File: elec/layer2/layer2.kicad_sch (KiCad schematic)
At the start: 24 parts, among them U4 DEV-15583

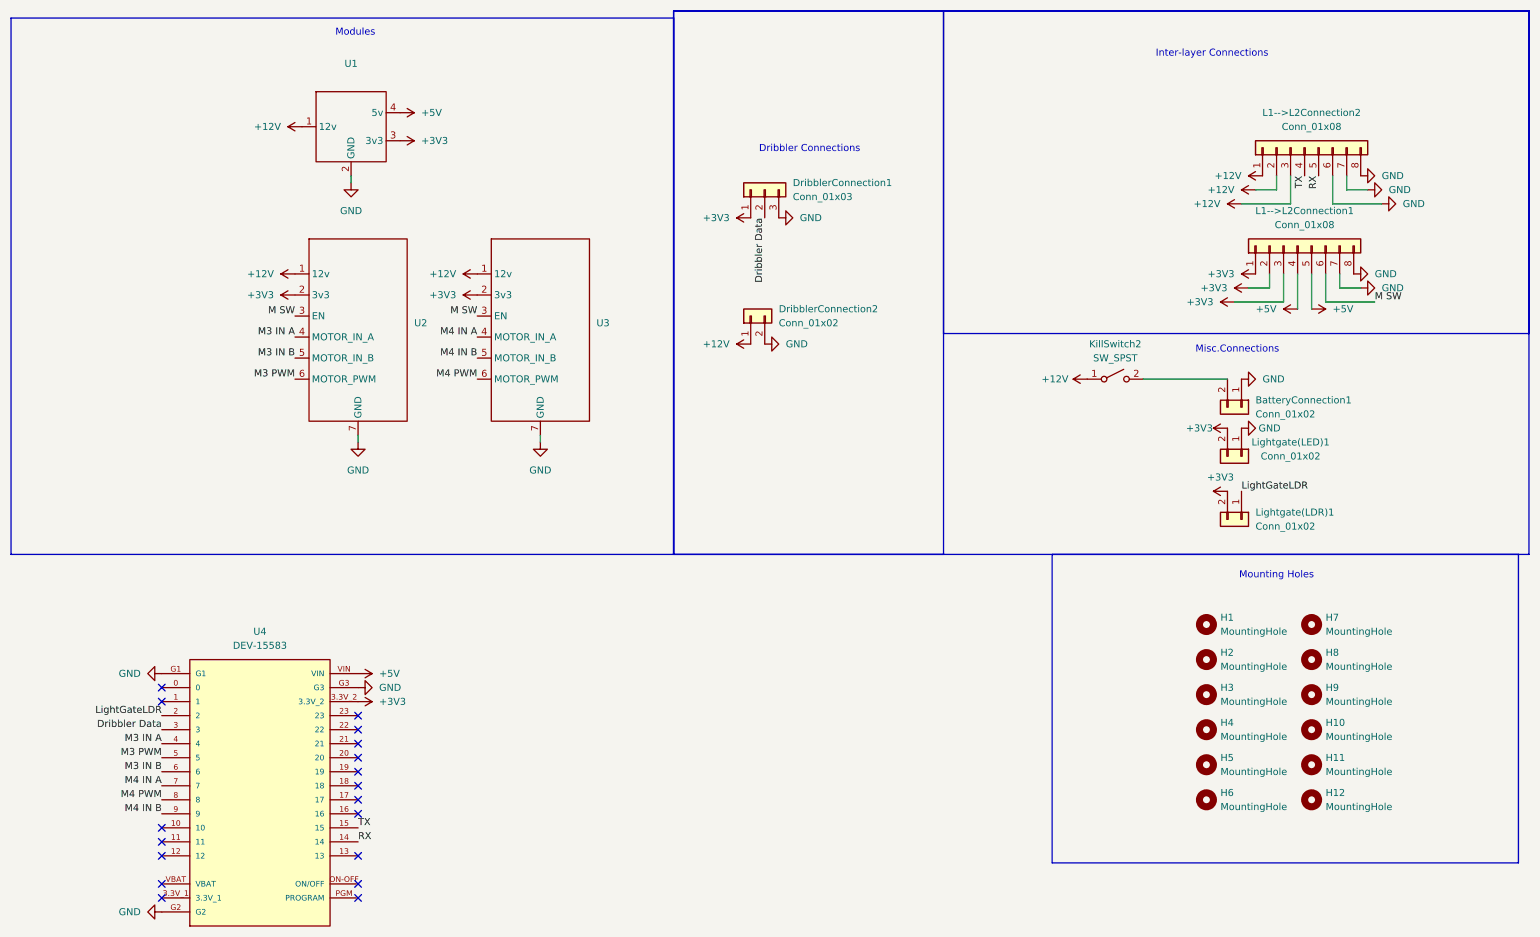
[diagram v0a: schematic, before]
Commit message: stuff
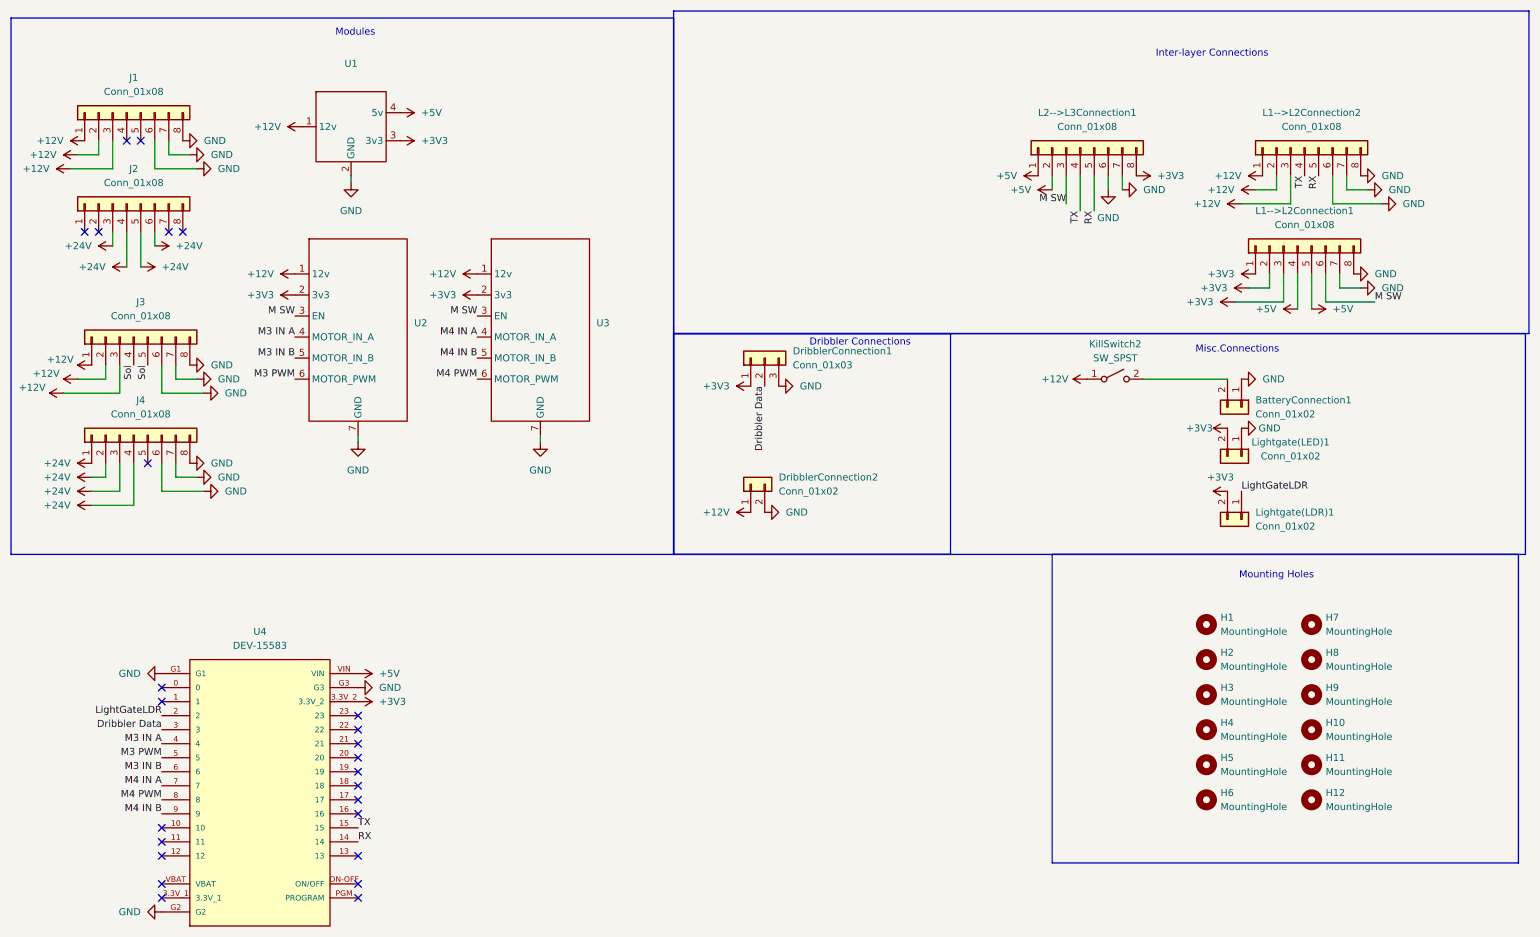
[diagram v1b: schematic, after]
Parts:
- added J1, J2, L2-->L3Connection1: Conn_01x08, Pinheaders:PinHeader_1x08_P2.54mm_Vertical, symbol Connector_Generic:Conn_01x08
- added J3, J4: Conn_01x08, Connector_PinSocket_2.54mm:PinSocket_1x08_P2.54mm_Vertical, symbol Connector_Generic:Conn_01x08
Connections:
- net +12V: now also J1.1 (Pin_1), J1.2 (Pin_2), J1.3 (Pin_3), J3.1 (Pin_1), J3.2 (Pin_2), J3.3 (Pin_3)
- net +3V3: now also L2-->L3Connection1.8 (Pin_8)
- net +5V: now also L2-->L3Connection1.1 (Pin_1), L2-->L3Connection1.2 (Pin_2)
- net GND: now also J1.6 (Pin_6), J1.7 (Pin_7), J1.8 (Pin_8), J3.6 (Pin_6), J3.7 (Pin_7), J3.8 (Pin_8), J4.6 (Pin_6), J4.7 (Pin_7), J4.8 (Pin_8), L2-->L3Connection1.6 (Pin_6), L2-->L3Connection1.7 (Pin_7)
- net M SW: now also L2-->L3Connection1.3 (Pin_3)
- net RX: now also L2-->L3Connection1.5 (Pin_5)
- net TX: now also L2-->L3Connection1.4 (Pin_4)
- new net +24V: J2.3 (Pin_3), J2.4 (Pin_4), J2.5 (Pin_5), J2.6 (Pin_6), J4.1 (Pin_1), J4.2 (Pin_2), J4.3 (Pin_3), J4.4 (Pin_4)
- new net Sol: J3.4 (Pin_4), J3.5 (Pin_5)
- no-connect marks 18 -> 25
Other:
- moved on the sheet: DribblerConnection1, DribblerConnection2
